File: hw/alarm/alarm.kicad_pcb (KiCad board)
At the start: 2 copper layers, 7.5 x 14.8 mm, 50 parts, among them IC1 DS3231S#T&R, IC2 TSOP38238, IC3 SHT40-BD1B-R2, IC4 23K256-I_SN, J1 4328, J2 SFV24R-4STBE1HLF, Q1 DMG2305UX-7, Q3 Si1308EDL-T1-GE3, U1 RaspberryPi_Pico, U2 PEC11R-4215F-S0024, U3 2462, U4 AS1115-BSST, U5 TDCR1060M

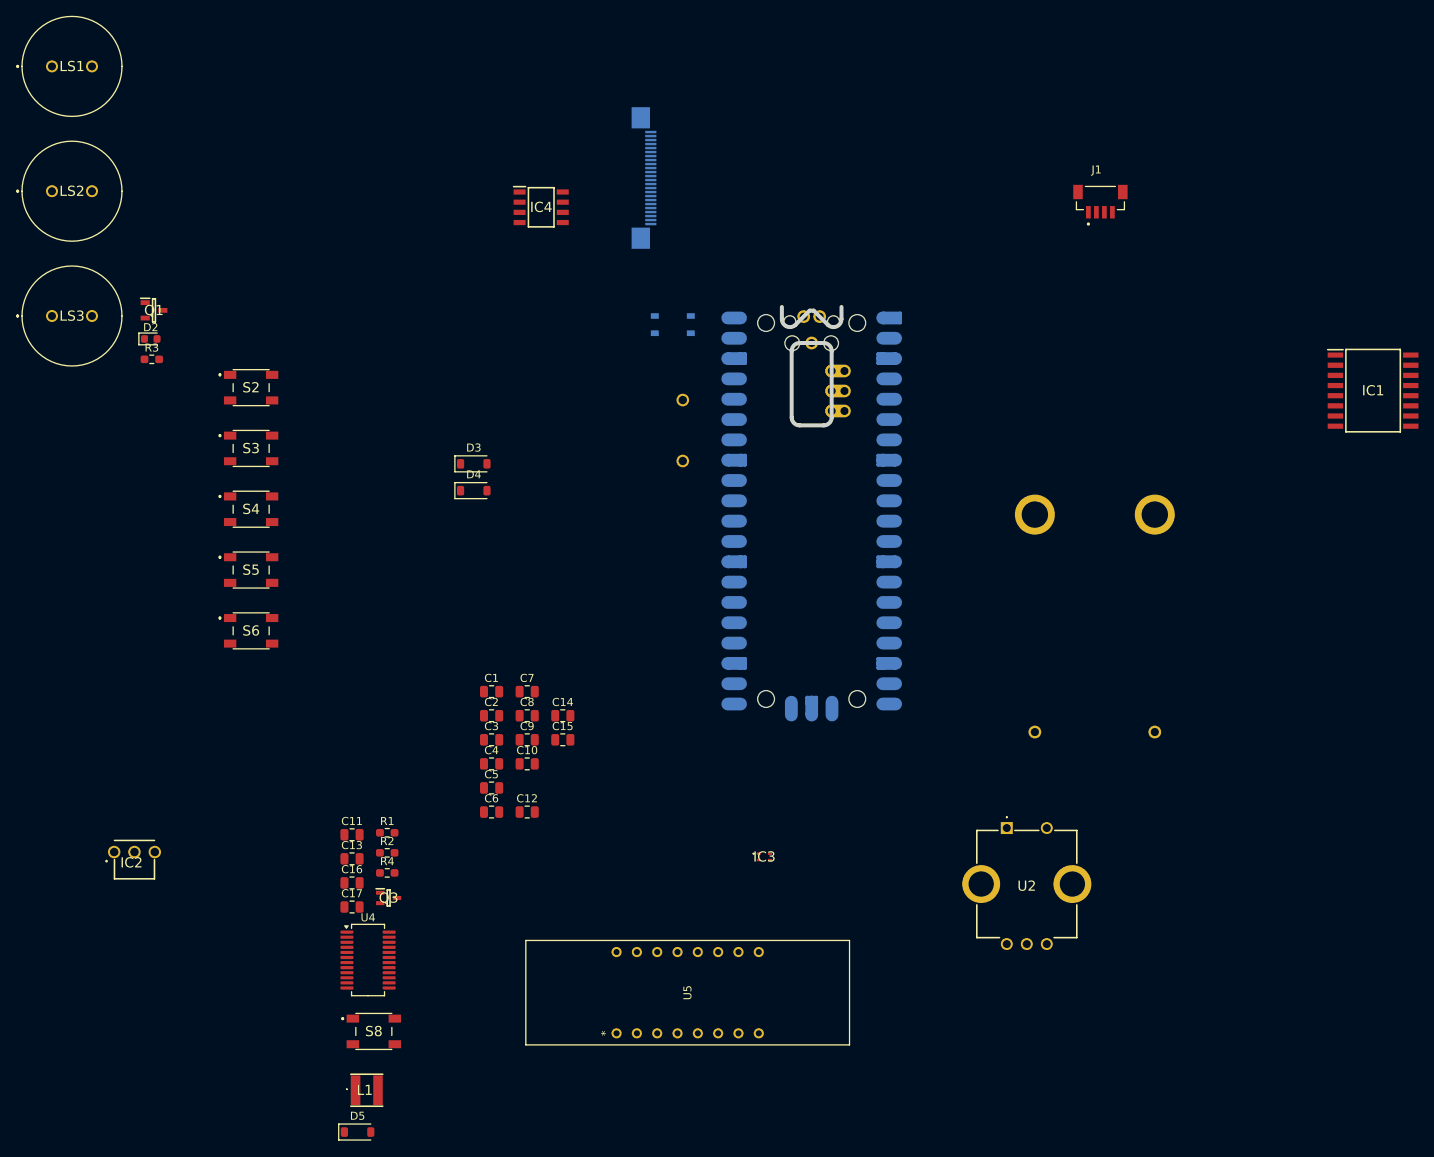
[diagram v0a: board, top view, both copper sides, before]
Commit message: Start board layout
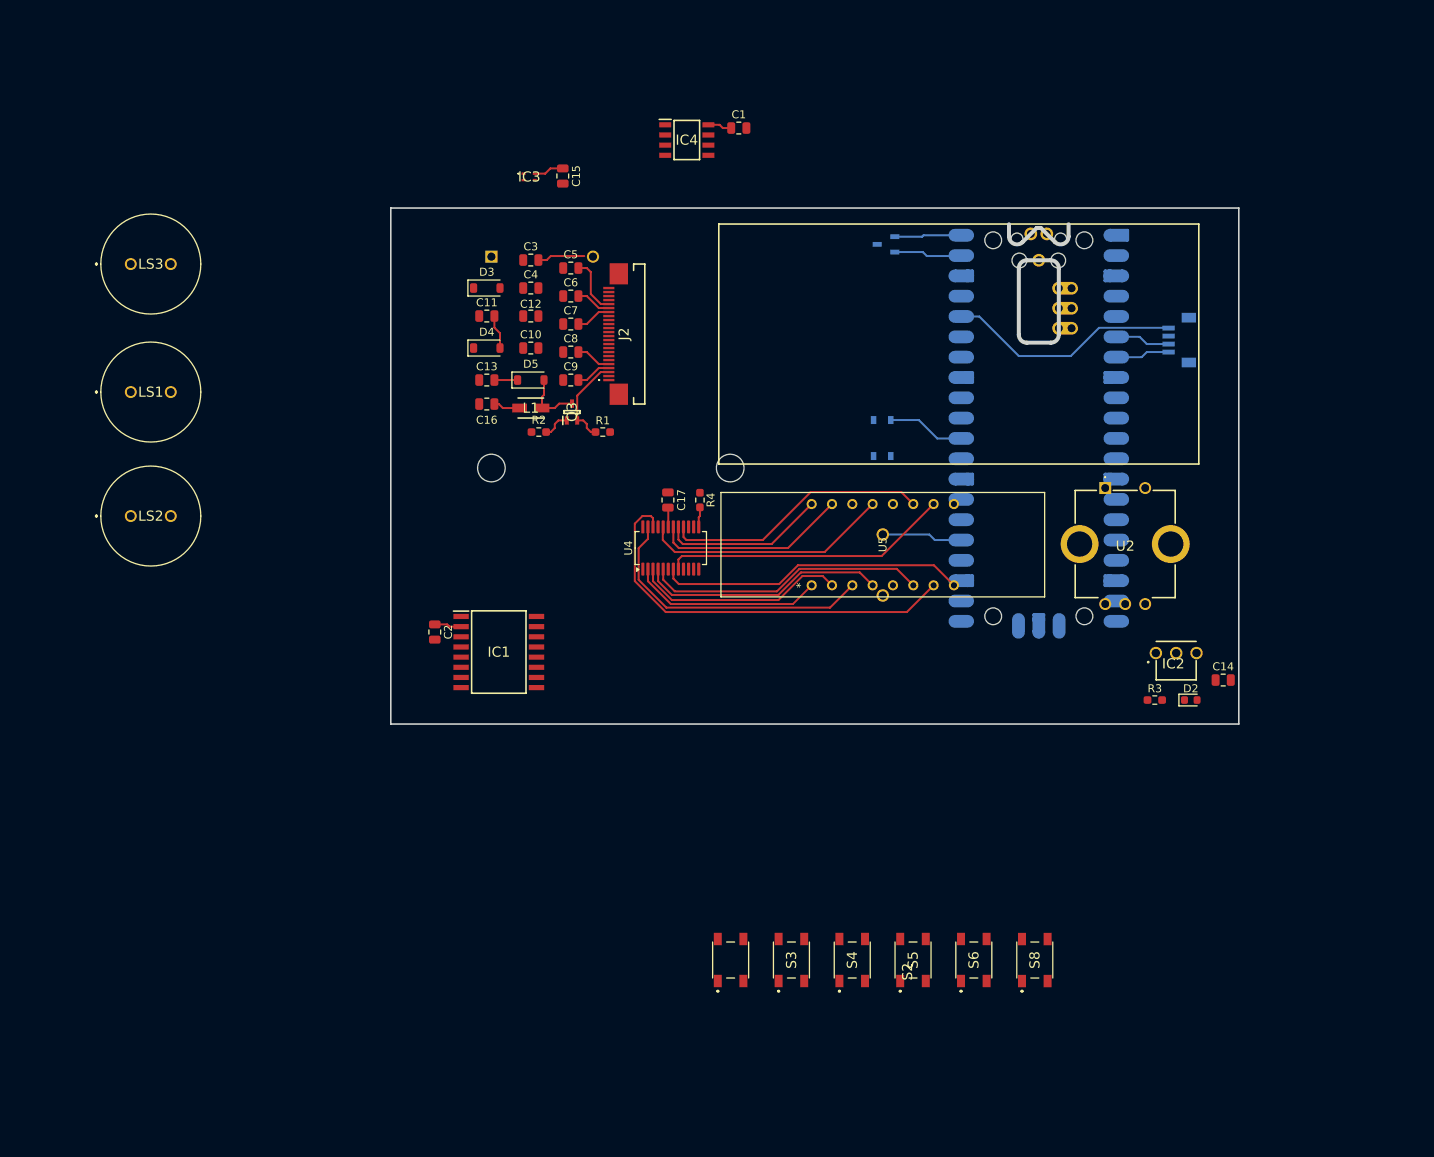
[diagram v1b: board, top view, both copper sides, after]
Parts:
- removed U3: 2462, SamacSys_Parts:2462
- added BT1: 2464, SamacSys_Parts:2464, B.Cu at (99.6, 71.6)
- C1, C11, C13, C14, C15, C17, C2, C3, C4, C5, C6, C7, C8, C9: value 0.1uF -> 1uF
- J1, Q1: moved to B.Cu
- J2: moved to F.Cu
- L1: value 10uH -> 68 uH; footprint SamacSys_Parts:NR4018T100M -> SamacSys_Parts:INDM3225X240N
- moved D2 137.6 mm to (187.0, 127.0)
- moved IC2 132.6 mm to (185.2, 119.7)
- moved R3 132.4 mm to (182.5, 127.0)
- moved IC1 114.1 mm to (100.5, 121.0)
- moved S6 99.3 mm to (159.9, 159.5), turned to 90 degrees
- moved D5 96.5 mm to (104.5, 87.0)
- moved S5 96.0 mm to (152.3, 159.5), turned to 90 degrees
- moved S4 93.9 mm to (144.7, 159.5), turned to 90 degrees
- moved S2 93.3 mm to (129.5, 159.5), turned to 90 degrees
- moved S3 93.0 mm to (137.1, 159.5), turned to 90 degrees
- moved Q1 91.9 mm to (148.9, 70.0), turned to 180 degrees
- moved IC3 89.9 mm to (104.3, 61.6)
- moved L1 87.7 mm to (104.5, 90.5)
- moved S8 83.1 mm to (167.5, 159.5), turned to 90 degrees
- moved C14 82.7 mm to (191.1, 124.5)
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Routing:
- net Net-(U4-SEGDP): track 0.00 -> 51.4 mm
- net +3.3V: track 0.00 -> 44.6 mm
- net Net-(U4-DIG4): track 0.00 -> 38.5 mm
- net Net-(U4-SEGD): track 0.00 -> 36.4 mm
- net Net-(U4-DIG5): track 0.00 -> 36.0 mm
- net Net-(U4-DIG3): track 0.00 -> 35.2 mm
- net Net-(U4-SEGF): track 0.00 -> 33.3 mm
- net Net-(U4-SEGC): track 0.00 -> 31.0 mm
- net Net-(U4-DIG2): track 0.00 -> 30.9 mm
- net Net-(U4-DIG1): track 0.00 -> 26.6 mm
- net Net-(U4-SEGG): track 0.00 -> 24.3 mm
- net Net-(U4-DIG0): track 0.00 -> 24.1 mm
- net Net-(U4-SEGB): track 0.00 -> 20.5 mm
- net /RESE: track 0.00 -> 11.5 mm
- net Net-(S7-NO): track 0.00 -> 10.9 mm
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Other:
- board size 7.5 x 14.8 mm -> 106 x 64.5 mm
